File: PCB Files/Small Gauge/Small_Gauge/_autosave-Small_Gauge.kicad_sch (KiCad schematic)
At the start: 1 part, among them U1 RP2040

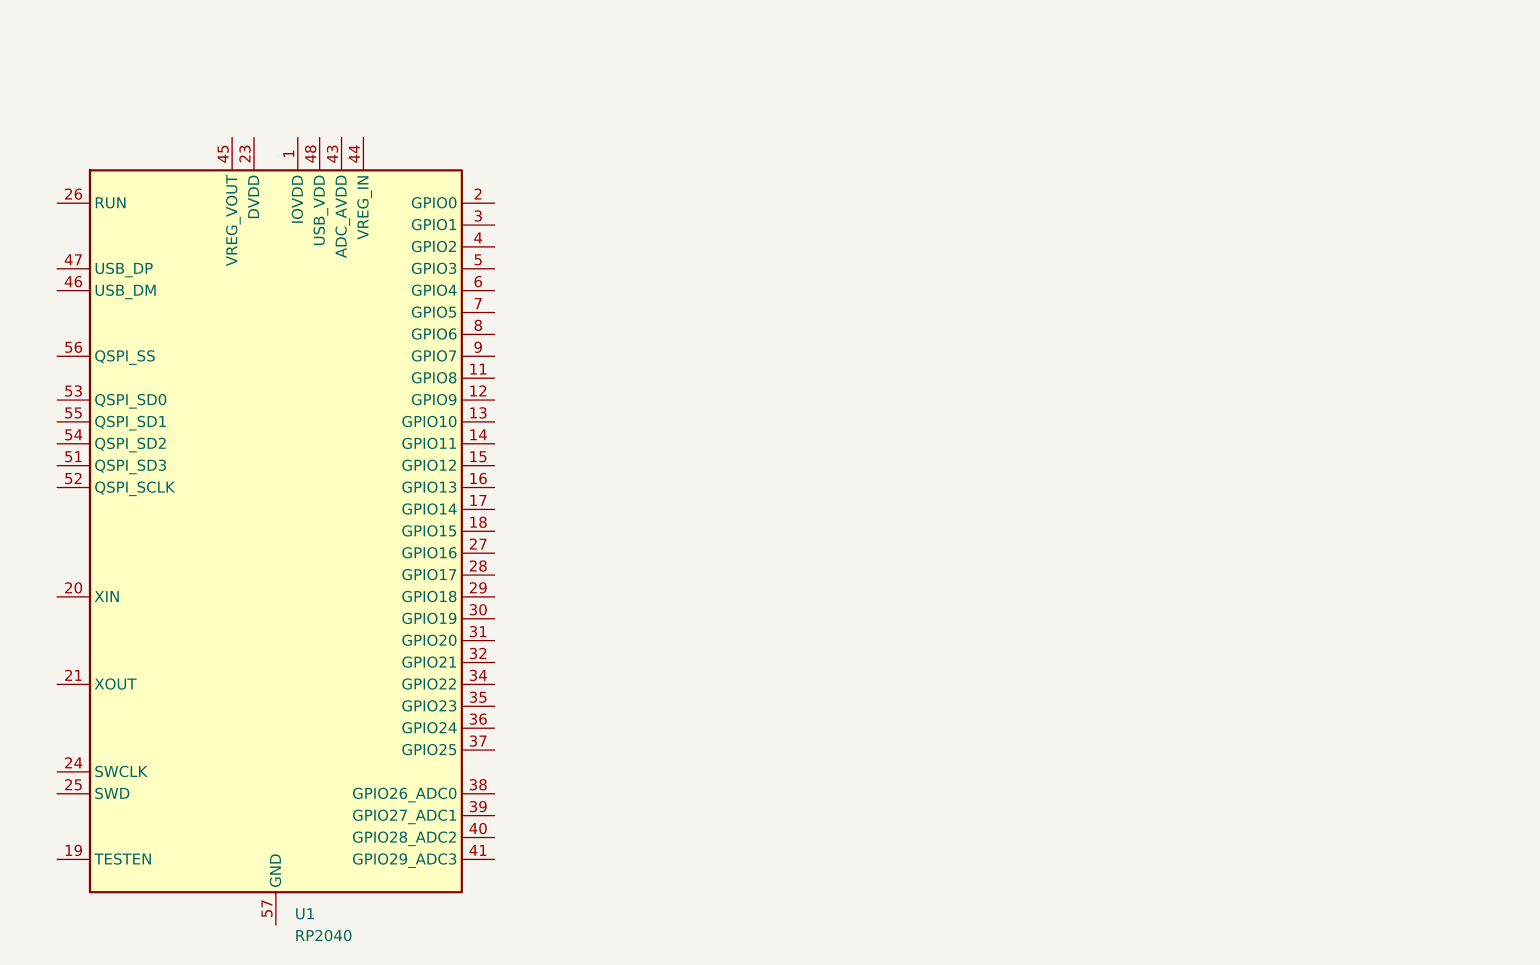
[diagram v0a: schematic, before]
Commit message: micro usb part
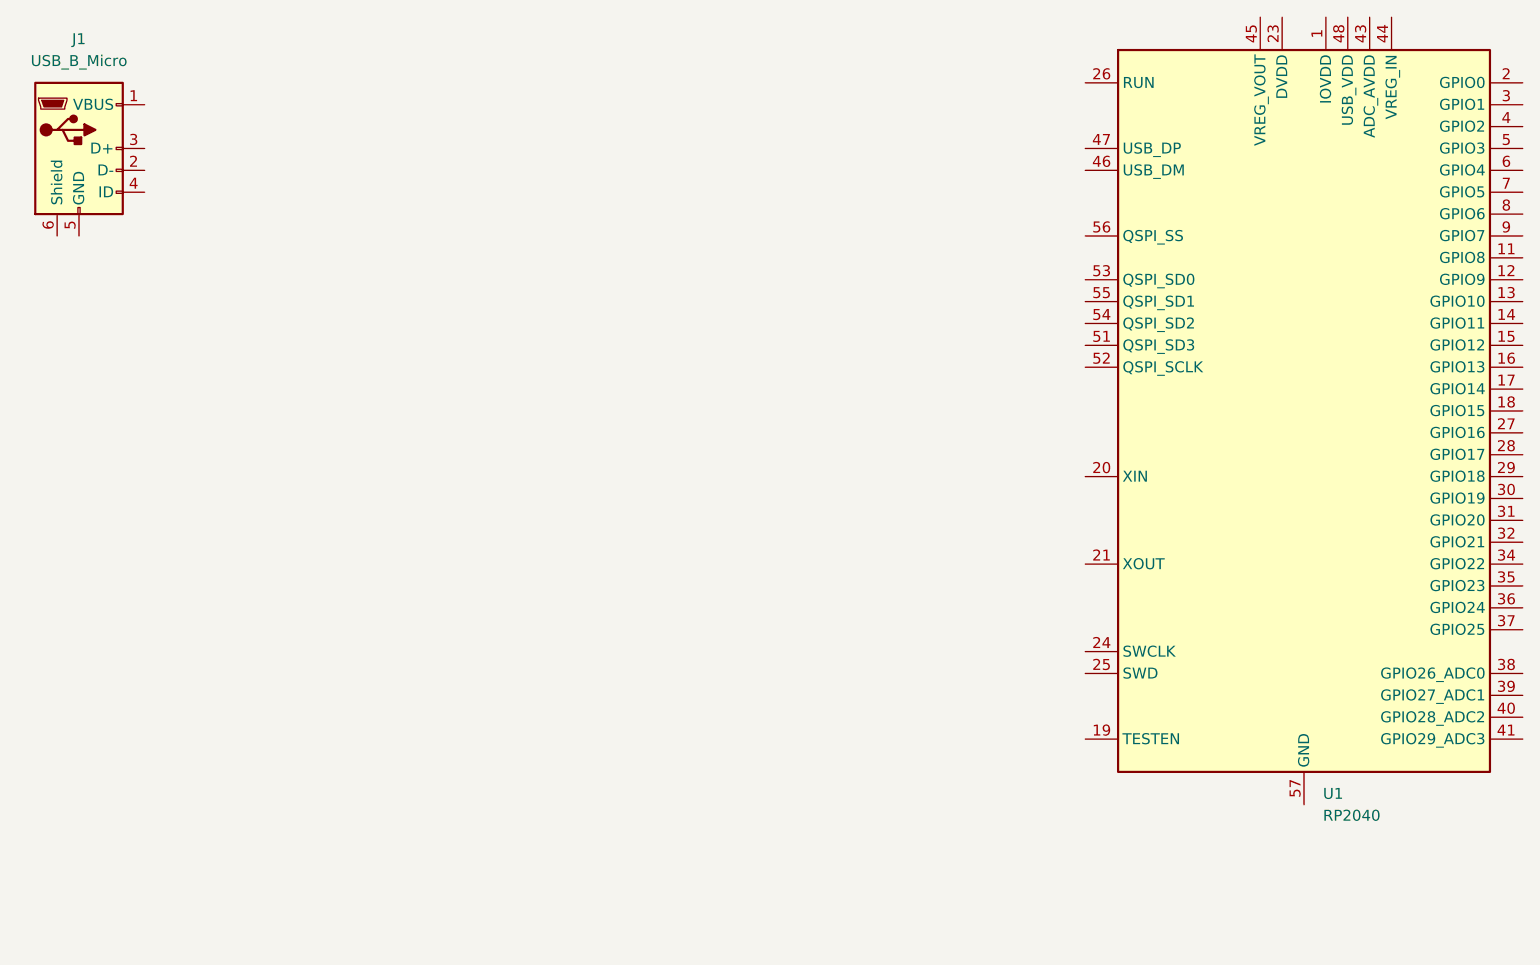
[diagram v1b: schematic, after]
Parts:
- added J1: USB_B_Micro, symbol Connector:USB_B_Micro
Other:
- moved on the sheet: U1
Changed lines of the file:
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@@
 (kicad_sch (version 20230121) (generator eeschema)
   (paper "A4")
-  (symbol (lib_id "MCU_RaspberryPi:RP2040") (at 60.96 83.82 0) (unit 1)
+  (symbol (lib_id "MCU_RaspberryPi:RP2040") (at 180.34 69.85 0) (unit 1)
     (in_bom yes) (on_board yes) (dnp no) (fields_autoplaced)
-    (property "Reference" "U1" (at 63.1541 128.27 0)
+    (property "Reference" "U1" (at 182.5341 114.3 0)
       (effects (font (size 1.27 1.27)) (justify left))
     )
-    (property "Value" "RP2040" (at 63.1541 130.81 0)
+    (property "Value" "RP2040" (at 182.5341 116.84 0)
       (effects (font (size 1.27 1.27)) (justify left))
     )
-    (property "Footprint" "Package_DFN_QFN:QFN-56-1EP_7x7mm_P0.4mm_EP3.2x3.2mm" (at 60.96 83.82 0)
+    (property "Footprint" "Package_DFN_QFN:QFN-56-1EP_7x7mm_P0.4mm_EP3.2x3.2mm" (at 180.34 69.85 0)
       (effects (font (size 1.27 1.27)) hide)
     )
-    (property "Datasheet" "https://datasheets.raspberrypi.com/rp2040/rp2040-datasheet.pdf" (at 60.96 83.82 0)
+    (property "Datasheet" "https://datasheets.raspberrypi.com/rp2040/rp2040-datasheet.pdf" (at 180.34 69.85 0)
       (effects (font (size 1.27 1.27)) hide)
     )
@@
         )
       )
+    )
+  )
+  (symbol (lib_id "Connector:USB_B_Micro") (at 38.1 39.37 0) (unit 1)
+    (in_bom yes) (on_board yes) (dnp no) (fields_autoplaced)
+    (property "Reference" "J1" (at 38.1 26.67 0)
+      (effects (font (size 1.27 1.27)))
+    )
+    (property "Value" "USB_B_Micro" (at 38.1 29.21 0)
+      (effects (font (size 1.27 1.27)))
+    )
+    (property "Footprint" "" (at 41.91 40.64 0)
+      (effects (font (size 1.27 1.27)) hide)
+    )
+    (property "Datasheet" "~" (at 41.91 40.64 0)
+      (effects (font (size 1.27 1.27)) hide)
+    )
+    (pin "1")
+    (pin "2")
+    (pin "3")
+    (pin "4")
+    (pin "5")
+    (pin "6")
+    (instances
+      (project "Small_Gauge"
+        (path "/49d5e9a8-2a01-4502-bd12-cb673056886d"
+          (reference "J1") (unit 1)
+        )
+      )
